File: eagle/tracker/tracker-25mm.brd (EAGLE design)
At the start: 57 x 26 mm, 45 parts, among them J1 BATT, J2 SHDN, M1 UBLOX-NEO-M8, M2 HOPE-RFM98W, U1 MS5637-02, U3 A25L010A, X1 MICROMATCH-4, X5 B3710U410

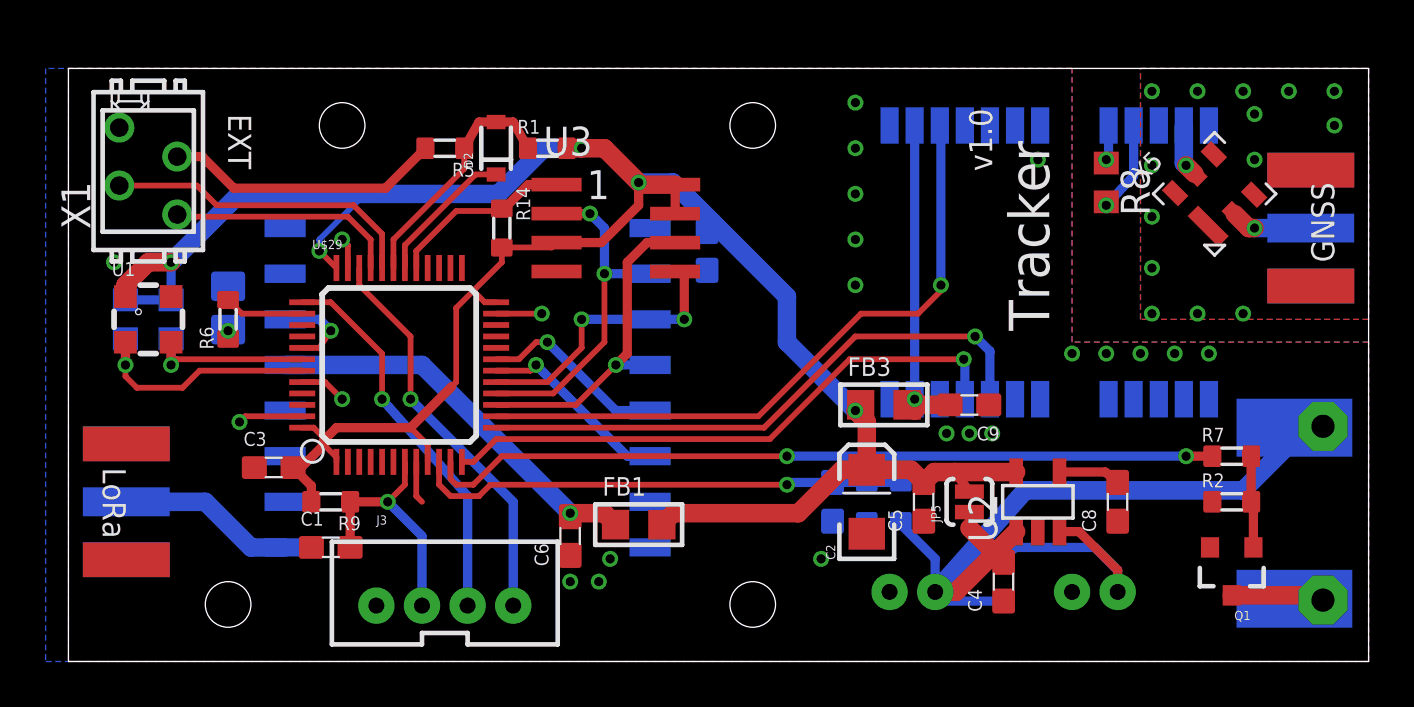
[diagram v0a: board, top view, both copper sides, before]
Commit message: Tracker ready for order
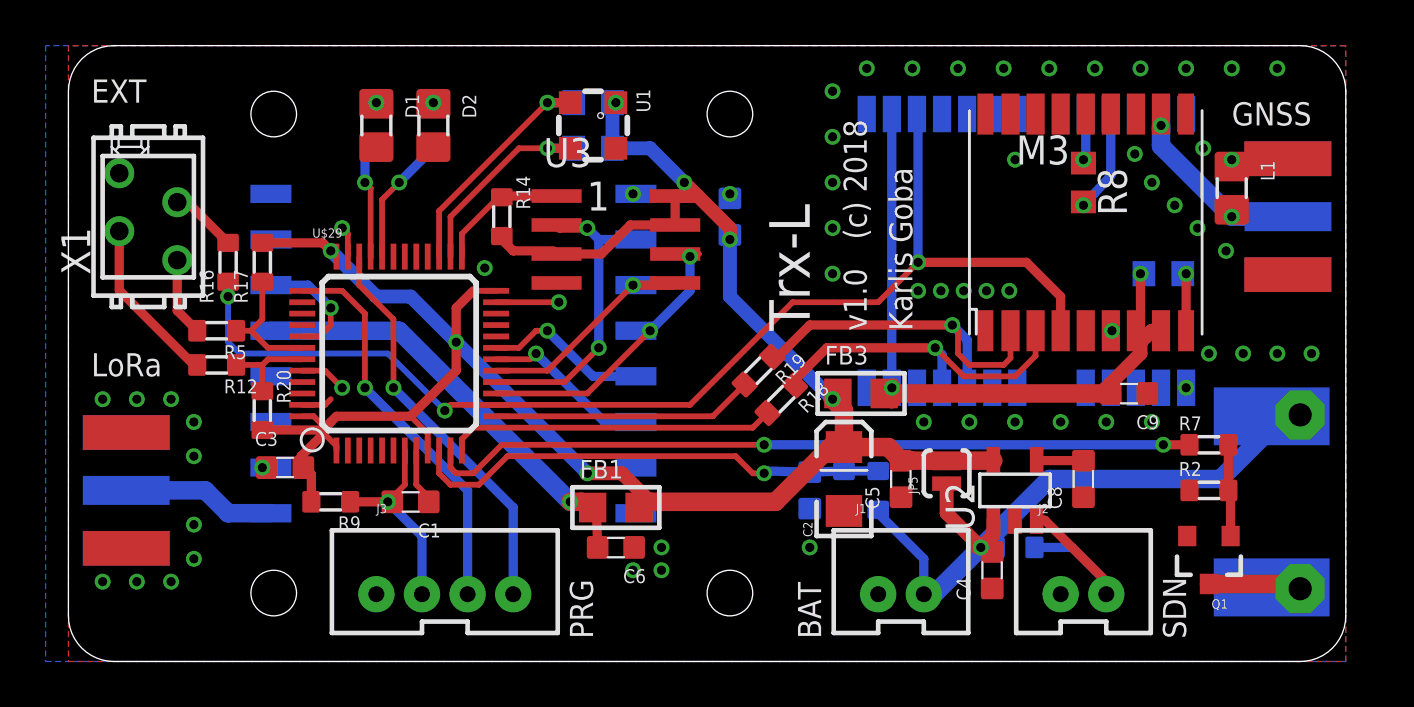
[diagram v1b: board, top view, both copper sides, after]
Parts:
- removed X5: B3710U410, kg-radio:DCC6C
- added L1: (no value), kg-generic:R0805
- added M3: UBLOX-MAX-M8, kg-modules:UBLOX-MAX
- added R12, R15, R16, R17, R18, R19, R20: (no value), kg-generic:R0603
- D2: device kg-generic:SOD-323 -> kg-generic:R0805
- R1: value (none) -> 3.3k; device kg-generic:R0603 -> rcl:R0603
- moved R1 27.6 mm to (48.0, 17.0), flipped to the bottom
- moved R4 22.6 mm to (23.0, 24.5), turned to 180 degrees
- moved U1 21.3 mm to (23.0, 23.5), turned to 270 degrees
- moved R3 20.0 mm to (23.0, 22.5), turned to 180 degrees
- moved R5 12.8 mm to (6.50, 14.5)
- moved M2 11.0 mm to (24.5, 20.5)
- moved R6 10.7 mm to (13.5, 23.5), flipped to the bottom, turned to 270 degrees
- moved D1 10.3 mm to (13.5, 23.5), flipped to the top, turned to 270 degrees
- moved C9 7.02 mm to (46.5, 11.8)
- moved C1 4.03 mm to (15.0, 7.00), turned to 180 degrees
- moved D2 2.93 mm to (16.0, 23.5), turned to 270 degrees
- moved C6 2.06 mm to (24.0, 5.00), turned to 180 degrees
- moved X1 2.00 mm to (3.50, 19.5)
- moved C7 1.80 mm to (29.0, 19.5), turned to 270 degrees
- moved C8 1.80 mm to (44.5, 8.00)
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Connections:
- removed net BUS: R5.2, X1.2
- removed net CMD1: U$29.32, X1.3
- removed net CMD2: U$29.33, X1.4
- removed net LED: R6.2, U$29.38
- new net LED1: R6.2, U$29.33
- new net LED2: R15.2, U$29.32
- new net N$20: R12.2, X1.3
- new net N$21: R5.2, X1.4
- new net N$22: D2.1, R15.1
- new net N$23: R18.2, U$29.12
- new net N$24: R16.2, X1.2
- new net N$25: R19.2, U$29.13
- net !FLASH_CS: now also U$29.25; no longer U$29.29
- net 3.3V: now also R17.2, R20.2; no longer R1.2
- net DBG_RX: now also R12.1, R20.1, U$29.43; no longer D2.A, R1.1, R5.1, U$29.31
- net DBG_TX: now also R17.1, R5.1, U$29.42; no longer D2.C, U$29.30
- net GND: now also D2.2, L1.1, M3.1, M3.10, M3.12, M3.6; no longer X5.1, X5.3, X5.4, X5.6
- net GPS_PPS: now also M3.4, R16.1
- net GPS_RXD: now also M3.2, R19.1; no longer U$29.13
- net GPS_TXD: now also M3.3, R18.1; no longer U$29.12
- net GPS_VCC: now also M3.7, M3.8, R1.2
- net N$5: now also L1.2, M1.11, M3.11; no longer X5.2
- net N$8: now also M3.9, R1.1; no longer M1.11, X5.5
- net SCL: now also U$29.26; no longer U$29.42
- net SDA: now also U$29.27; no longer U$29.43
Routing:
- net GPS_PPS: track 29.9 -> 52.6 mm, vias 1 -> 3
- net GPS_VCC: track 14.8 -> 30.2 mm, vias 1 -> 2
- net N$23: track 0.00 -> 14.4 mm
- net CMD1: track 13.9 -> 0.00 mm
- net BUS: track 12.2 -> 0.00 mm
- net N$25: track 0.00 -> 11.5 mm
- net GPS_TXD: track 25.6 -> 15.3 mm
- net CMD2: track 10.2 -> 0.00 mm
- net 3.3V: track 104.7 -> 94.6 mm, vias 5 -> 7
- net GPS_RXD: track 25.7 -> 16.8 mm
- net N$20: track 0.00 -> 7.37 mm
- net DBG_RX: track 10.7 -> 4.15 mm
- net N$5: track 3.59 -> 9.60 mm, vias 1 -> 2
- net LED2: track 0.00 -> 5.83 mm, vias 0 -> 1
- net V_BATT: track 38.6 -> 33.0 mm, vias 0 -> 1
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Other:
- board size 57 x 26 mm -> 56 x 27 mm
- board text added: "(c) 2018"
- board text added: "Karlis Goba"
- board text added: "PRG"
- board text added: "Trx-L"
- board text removed: "PROG"
- board text removed: "Tracker"
